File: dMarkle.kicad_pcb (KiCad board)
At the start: 2 copper layers, 99.7 x 75 mm, 61 parts, among them SW1 SW_Choice, U1 74LS125, U10 INND-TS30RCB, U2 74HC4511, U3 Pico, U4 INND-TS30RCB, U5 74LS125, U6 74LS125, U7 74HC4511, U8 74HC4511, U9 INND-TS30RCB

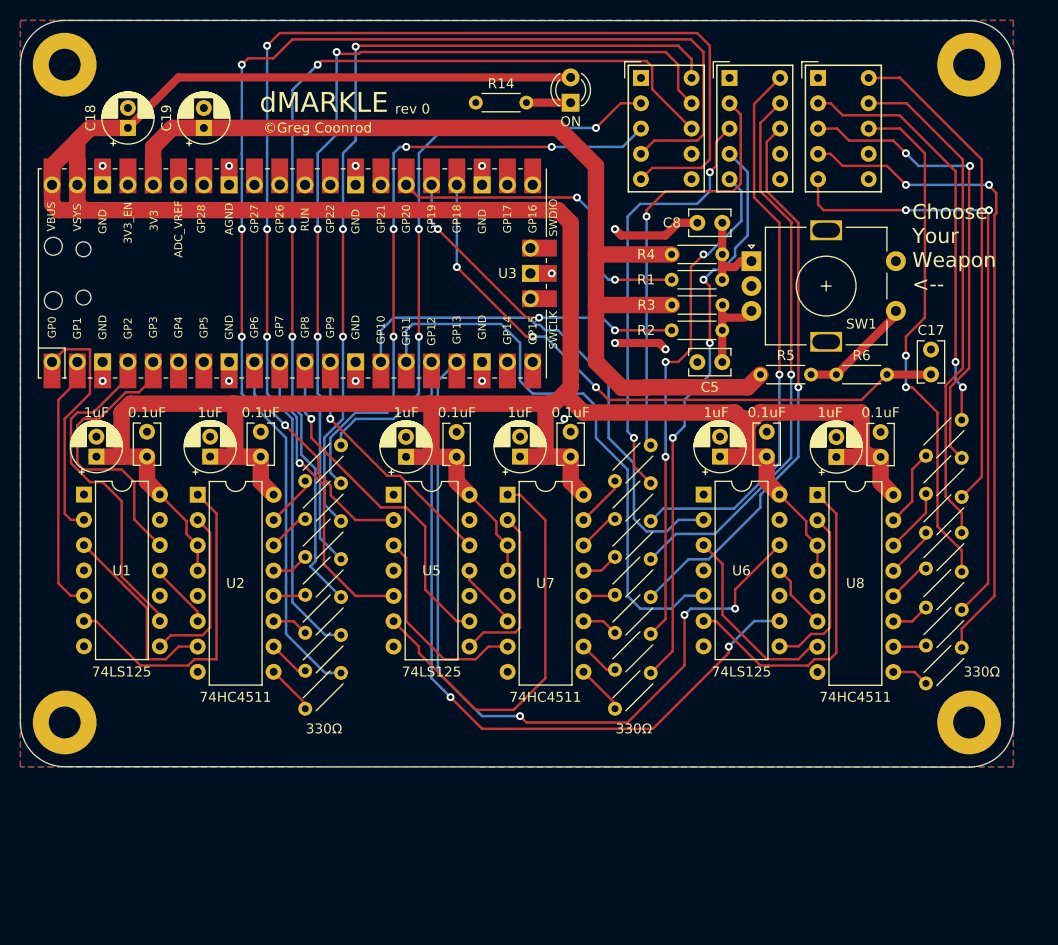
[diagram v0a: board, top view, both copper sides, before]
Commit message: Rev 0.1
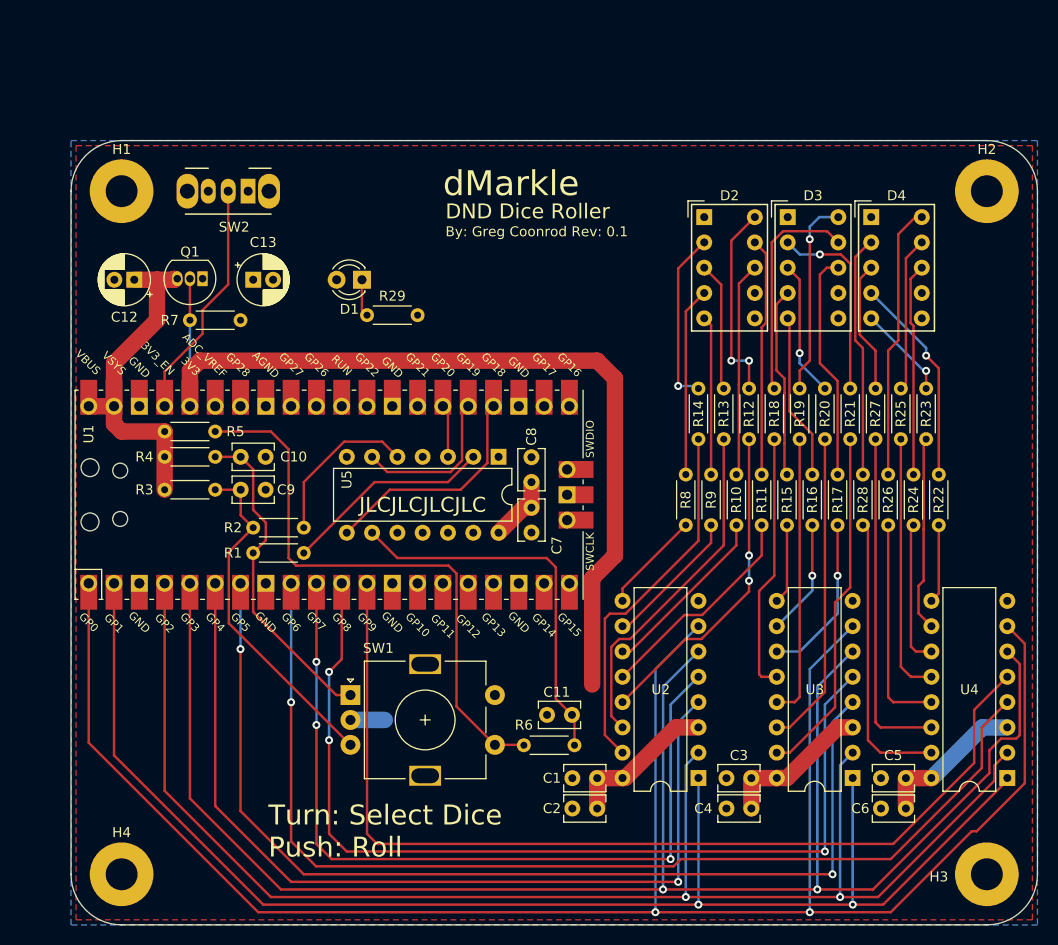
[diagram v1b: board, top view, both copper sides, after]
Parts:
- removed C14, C17: 0u1, Capacitor_THT:C_Rect_L4.0mm_W2.5mm_P2.50mm
- removed C18, C19: 10u, Capacitor_THT:CP_Radial_D5.0mm_P2.00mm
- removed U10, U9: INND-TS30RCB, Display_7Segment:HDSP-A151
- removed U6: 74LS125, Package_DIP:DIP-14_W7.62mm
- removed U7, U8: 74HC4511, Package_DIP:DIP-16_W7.62mm
- added D2: INND-TS30RCB, Display_7Segment:HDSP-A151, F.Cu at (152.5, 81.3)
- added D3: INND-TS30RCB, Display_7Segment:HDSP-A151, F.Cu at (160.9, 81.3)
- added D4: INND-TS30RCB, Display_7Segment:HDSP-A151, F.Cu at (169.2, 81.3)
- added Q1: 2N7000, Package_TO_SOT_THT:TO-92_Inline, F.Cu at (102.1, 87.5)
- added R29: 300, Resistor_THT:R_Axial_DIN0204_L3.6mm_D1.6mm_P5.08mm_Horizontal, F.Cu at (118.6, 91.2)
- added SW2: SW_EN, Button_Switch_THT:SW_CuK_OS102011MA1QN1_SPDT_Angled, F.Cu at (106.7, 78.7)
- C1, C3: footprint Capacitor_THT:CP_Radial_D5.0mm_P2.00mm -> Capacitor_THT:C_Rect_L4.0mm_W2.5mm_P2.50mm
- C10: value 0u1 -> 10n
- C11, C6: value 1u -> 0u1; footprint Capacitor_THT:CP_Radial_D5.0mm_P2.00mm -> Capacitor_THT:C_Rect_L4.0mm_W2.5mm_P2.50mm
- C12: value 0u1 -> 10u; footprint Capacitor_THT:C_Rect_L4.0mm_W2.5mm_P2.50mm -> Capacitor_THT:CP_Radial_D5.0mm_P2.00mm
- C13: value 1u -> 10u
- C5: value 10n -> 1u
- C7: value 0u1 -> 1u
- C8: value 10n -> 0u1
- C9: value 1u -> 10n; footprint Capacitor_THT:CP_Radial_D5.0mm_P2.00mm -> Capacitor_THT:C_Rect_L4.0mm_W2.5mm_P2.50mm
- R14: value 300 -> 330
- R7: value 330 -> 10k
- U1: value 74LS125 -> Pico; footprint Package_DIP:DIP-14_W7.62mm -> MCU_RaspberryPi_and_Boards:RPi_Pico_SMD_TH
- U3: value Pico -> 74HC4511; footprint MCU_RaspberryPi_and_Boards:RPi_Pico_SMD_TH -> Package_DIP:DIP-16_W7.62mm
- U4: value INND-TS30RCB -> 74HC4511; footprint Display_7Segment:HDSP-A151 -> Package_DIP:DIP-16_W7.62mm
- moved H4 117.7 mm to (94.0, 147.3)
- moved H2 106.8 mm to (180.8, 78.7)
- moved U4 79.3 mm to (182.9, 137.7), turned to 180 degrees
- moved U3 75.7 mm to (167.4, 137.7), turned to 180 degrees
- moved C12 65.9 mm to (95.2, 87.6), turned to 180 degrees
- moved C3 63.2 mm to (157.2, 137.7), turned to 180 degrees
- moved C6 61.4 mm to (172.7, 140.7), turned to 180 degrees
- moved C13 61.2 mm to (107.2, 87.6), turned to 0 degrees
- moved C4 60.6 mm to (157.2, 140.7), turned to 180 degrees
- moved R5 60.1 mm to (98.3, 102.9)
- moved C1 59.8 mm to (141.7, 137.7), turned to 180 degrees
- moved SW1 59.3 mm to (117.0, 129.3)
- moved U2 57.8 mm to (151.9, 137.7), turned to 180 degrees
- moved C2 57.4 mm to (141.7, 140.7), turned to 180 degrees
- moved R4 54.8 mm to (98.3, 105.4)
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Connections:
- net /D1G renamed Net-(R13-Pad1)
- C1 pad 1: +5V -> +3.3V
- C10 pad 1: +5V -> Net-(C10-Pad1)
- C11 pad 1: +5V -> Net-(C11-Pad1)
- C13 pad 1: +5V -> +3.3V
- C2 pad 1: +5V -> +3.3V
- C3 pad 1: +5V -> +3.3V
- C4 pad 1: +5V -> +3.3V
- C5 pad 1: Net-(C5-Pad1) -> +3.3V
- C6 pad 1: +5V -> +3.3V
- C7 pad 1: +5V -> +3.3V
- C8 pad 1: Net-(C8-Pad1) -> +3.3V
- C9 pad 1: +5V -> Net-(C9-Pad1)
- D1 pad 2: +5V -> +3.3V
- R1 pad 1: /R_CLK -> Net-(R1-Pad1)
- R1 pad 2: Net-(C8-Pad1) -> Net-(C10-Pad1)
- R10 pad 1: /D1D -> Net-(R10-Pad1)
- R10 pad 2: /D1Dr -> Net-(D2-Pad8)
- R11 pad 1: /D1E -> Net-(R11-Pad1)
- R11 pad 2: /D1Er -> Net-(D2-Pad9)
- R12 pad 1: /D1F -> Net-(R12-Pad1)
- R12 pad 2: /D1Fr -> Net-(D2-Pad10)
- R13 pad 2: /D1Gr -> Net-(D2-Pad3)
- R14 pad 1: Net-(D1-Pad1) -> Net-(R14-Pad1)
- R14 pad 2: GND -> Net-(D2-Pad2)
- R15 pad 1: /D2A -> Net-(U3-Pad9)
- R15 pad 2: /D2Ar -> Net-(D3-Pad4)
- R16 pad 1: /D2B -> Net-(U3-Pad10)
- R16 pad 2: /D2Br -> Net-(D3-Pad5)
- R17 pad 1: /D2C -> Net-(U3-Pad11)
- R17 pad 2: /D2Cr -> Net-(D3-Pad8)
- R18 pad 1: /D2D -> Net-(U3-Pad12)
- R18 pad 2: /D2Dr -> Net-(D3-Pad9)
- R19 pad 1: /D2E -> Net-(U3-Pad13)
- R19 pad 2: /D2Er -> Net-(D3-Pad10)
- R2 pad 1: /R_DT -> Net-(R2-Pad1)
- R2 pad 2: Net-(C5-Pad1) -> Net-(C9-Pad1)
- R20 pad 1: /D2F -> Net-(U3-Pad14)
- R20 pad 2: /D2Fr -> Net-(D3-Pad3)
- R21 pad 1: /D2G -> Net-(U3-Pad15)
- R21 pad 2: /D2Gr -> Net-(D3-Pad2)
- R22 pad 1: /D3A -> Net-(U4-Pad9)
- R22 pad 2: /D3Ar -> Net-(D4-Pad4)
- R23 pad 1: /D3B -> Net-(U4-Pad10)
- R23 pad 2: /D3Br -> Net-(D4-Pad5)
- R24 pad 1: /D3C -> Net-(U4-Pad11)
- R24 pad 2: /D3Cr -> Net-(D4-Pad8)
- R25 pad 1: /D3D -> Net-(U4-Pad12)
- R25 pad 2: /D3Dr -> Net-(D4-Pad9)
- R26 pad 1: /D3E -> Net-(U4-Pad13)
- R26 pad 2: /D3Er -> Net-(D4-Pad10)
- R27 pad 1: /D3F -> Net-(U4-Pad14)
- R27 pad 2: /D3Fr -> Net-(D4-Pad3)
- R28 pad 1: /D3G -> Net-(U4-Pad15)
- R28 pad 2: /D3Gr -> Net-(D4-Pad2)
- R3 pad 1: +3.3V -> +5V
- R3 pad 2: Net-(C5-Pad1) -> Net-(C9-Pad1)
- R4 pad 1: +3.3V -> +5V
- R4 pad 2: Net-(C8-Pad1) -> Net-(C10-Pad1)
- R5 pad 1: +3.3V -> +5V
- R6 pad 2: /R_~{SW} -> Net-(C11-Pad1)
- R7 pad 1: /D1A -> +3.3V
- R7 pad 2: /D1Ar -> GND
- R8 pad 1: /D1B -> Net-(R8-Pad1)
- R8 pad 2: /D1Br -> Net-(D2-Pad4)
- R9 pad 1: /D1C -> Net-(R9-Pad1)
- R9 pad 2: /D1Cr -> Net-(D2-Pad5)
- SW1 pad A: Net-(C8-Pad1) -> Net-(C10-Pad1)
- SW1 pad B: Net-(C5-Pad1) -> Net-(C9-Pad1)
- U1 pad 1: GND -> /D0
- U1 pad 10: GND -> /~{LE}1
- U1 pad 11: Net-(U1-Pad11) -> /~{LE}2
- U1 pad 12: /DIG0_3 -> /~{LE}3
- U1 pad 14: +5V -> unconnected-(U1-Pad14)
- U1 pad 2: /DIG0_0 -> /D1
- U1 pad 3: Net-(U1-Pad3) -> GND
- U1 pad 4: GND -> /D2
- U1 pad 5: /DIG0_1 -> /D3
- U1 pad 6: Net-(U1-Pad6) -> /~{BL}1
- U1 pad 7: GND -> /~{BL}2
- U1 pad 8: Net-(U1-Pad8) -> GND
- U1 pad 9: /DIG0_2 -> /~{BL}3
- U2 pad 1: Net-(U1-Pad6) -> /D1
- U2 pad 10: /D1D -> Net-(R9-Pad1)
- U2 pad 11: /D1C -> Net-(R10-Pad1)
- U2 pad 12: /D1B -> Net-(R11-Pad1)
- U2 pad 13: /D1A -> Net-(R12-Pad1)
- U2 pad 15: /D1F -> Net-(R14-Pad1)
- U2 pad 16: +5V -> +3.3V
- U2 pad 2: Net-(U1-Pad8) -> /D2
- U2 pad 3: +5V -> +3.3V
- U2 pad 4: +5V -> /~{BL}1
- U2 pad 5: GND -> /~{LE}1
- U2 pad 6: Net-(U1-Pad11) -> /D3
- U2 pad 7: Net-(U1-Pad3) -> /D0
- U2 pad 9: /D1E -> Net-(R8-Pad1)
- U3 pad 1: /DIG0_0 -> /D1
- U3 pad 10: /DIG1_1 -> Net-(U3-Pad10)
- U3 pad 11: /DIG1_2 -> Net-(U3-Pad11)
- U3 pad 12: /DIG1_3 -> Net-(U3-Pad12)
- U3 pad 13: GND -> Net-(U3-Pad13)
- U3 pad 14: /DIG2_0 -> Net-(U3-Pad14)
- U3 pad 15: /DIG2_1 -> Net-(U3-Pad15)
- U3 pad 16: /DIG2_2 -> +3.3V
- U3 pad 2: /DIG0_1 -> /D2
- U3 pad 3: GND -> +3.3V
- U3 pad 4: /DIG0_2 -> /~{BL}2
- U3 pad 5: /DIG0_3 -> /~{LE}2
- U3 pad 6: unconnected-(U3-Pad6) -> /D3
- U3 pad 7: unconnected-(U3-Pad7) -> /D0
- U3 pad 9: /DIG1_0 -> Net-(U3-Pad9)
- U4 pad 1: GND -> /D1
- U4 pad 10: /D1Ar -> Net-(U4-Pad10)
- U4 pad 2: /D1Fr -> /D2
- U4 pad 3: /D1Gr -> +3.3V
- U4 pad 4: /D1Er -> /~{BL}3
- U4 pad 5: /D1Dr -> /~{LE}3
- U4 pad 6: GND -> /D3
- U4 pad 7: unconnected-(U4-Pad7) -> /D0
- U4 pad 8: /D1Cr -> GND
- U4 pad 9: /D1Br -> Net-(U4-Pad9)
- U5 pad 11: Net-(U5-Pad11) -> unconnected-(U5-Pad11)
- U5 pad 12: /DIG1_3 -> unconnected-(U5-Pad12)
- U5 pad 13: GND -> unconnected-(U5-Pad13)
- U5 pad 14: +5V -> +3.3V
- U5 pad 2: /DIG1_0 -> Net-(R1-Pad1)
- U5 pad 3: Net-(U5-Pad3) -> /R_CLK
- U5 pad 5: /DIG1_1 -> Net-(R2-Pad1)
- U5 pad 6: Net-(U5-Pad6) -> /R_DT
- U5 pad 8: Net-(U5-Pad8) -> /R_~{SW}
- U5 pad 9: /DIG1_2 -> Net-(C11-Pad1)
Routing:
- net +5V: track 331.1 -> 34.2 mm
- net /D0: track 0.00 -> 199.9 mm, vias 0 -> 2
- net /D3: track 0.00 -> 176.1 mm, vias 0 -> 2
- net /D2: track 0.00 -> 146.8 mm, vias 0 -> 2
- net /D1: track 0.00 -> 144.0 mm, vias 0 -> 2
- net /D1Er: track 129.4 -> 0.00 mm, vias 3 -> 0
- net /D1Dr: track 127.8 -> 0.00 mm, vias 3 -> 0
- net /~{BL}3: track 0.00 -> 108.1 mm, vias 0 -> 1
- net /~{BL}2: track 0.00 -> 103.1 mm, vias 0 -> 2
- net /~{LE}3: track 0.00 -> 99.9 mm
- net /D1Cr: track 98.8 -> 0.00 mm, vias 3 -> 0
- net /~{LE}2: track 0.00 -> 94.9 mm, vias 0 -> 3
- net /D1Br: track 92.1 -> 0.00 mm, vias 3 -> 0
- net /~{BL}1: track 0.00 -> 90.9 mm, vias 0 -> 1
- net /D1Ar: track 85.8 -> 0.00 mm, vias 3 -> 0
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- added copper zone on F.Cu, net +3.3V
- removed copper zone on F.Cu, net GND
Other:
- board size 99.7 x 75 mm -> 97 x 78.7 mm
- rule pad_to_mask_clearance: 0.05 -> 0
- board text added: "By: Greg Coonrod Rev: 0.1"
- board text added: "DND Dice Roller"
- board text added: "JLCJLCJLCJLC"
- board text added: "Turn: Select Dice Push: Roll"
- board text added: "dMarkle"
- board text removed: "0.1uF"
- board text removed: "1uF"
- board text removed: "330Ω"
- board text removed: "Choose Your Weapon <--"
- board text removed: "ON"
- board text removed: "dMARKLE"
- board text removed: "rev 0"
- board text removed: "©Greg Coonrod"
